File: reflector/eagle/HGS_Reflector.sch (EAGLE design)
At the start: 22 parts, among them J1 U.FL, U1 TQP3M9037, U2 TQP3M903X, U3 LP2985XX-N

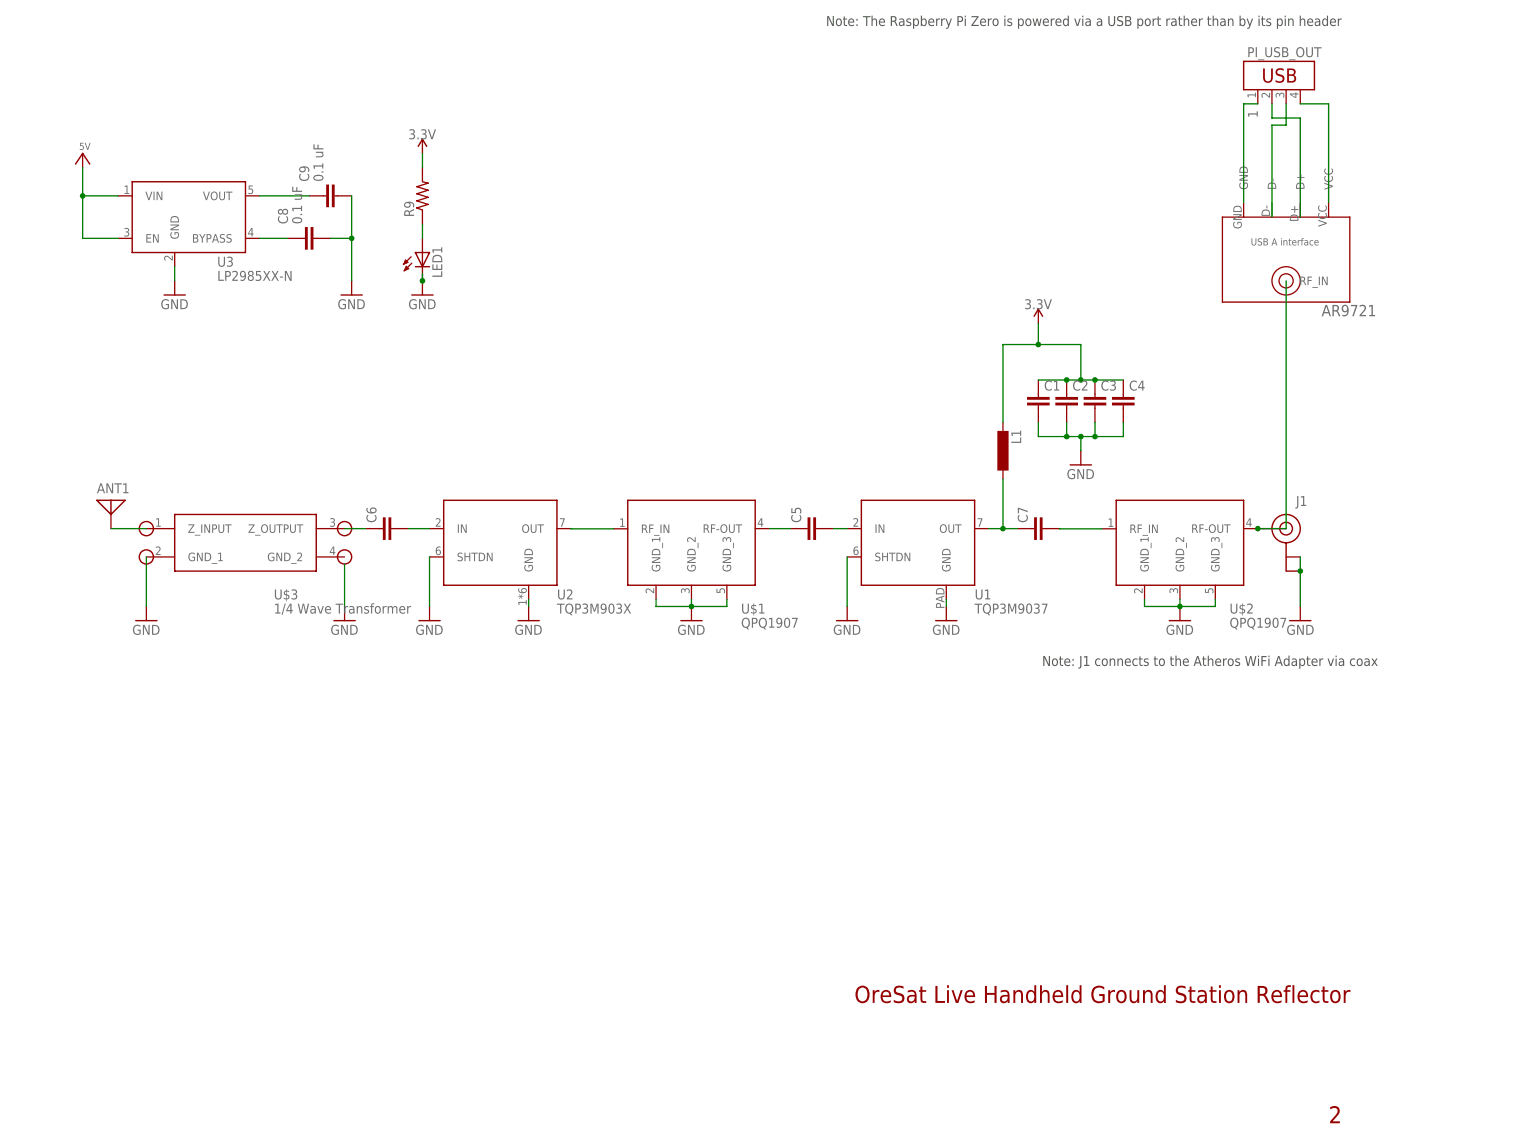
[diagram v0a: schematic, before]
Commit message: Schematic, board and BOM updates
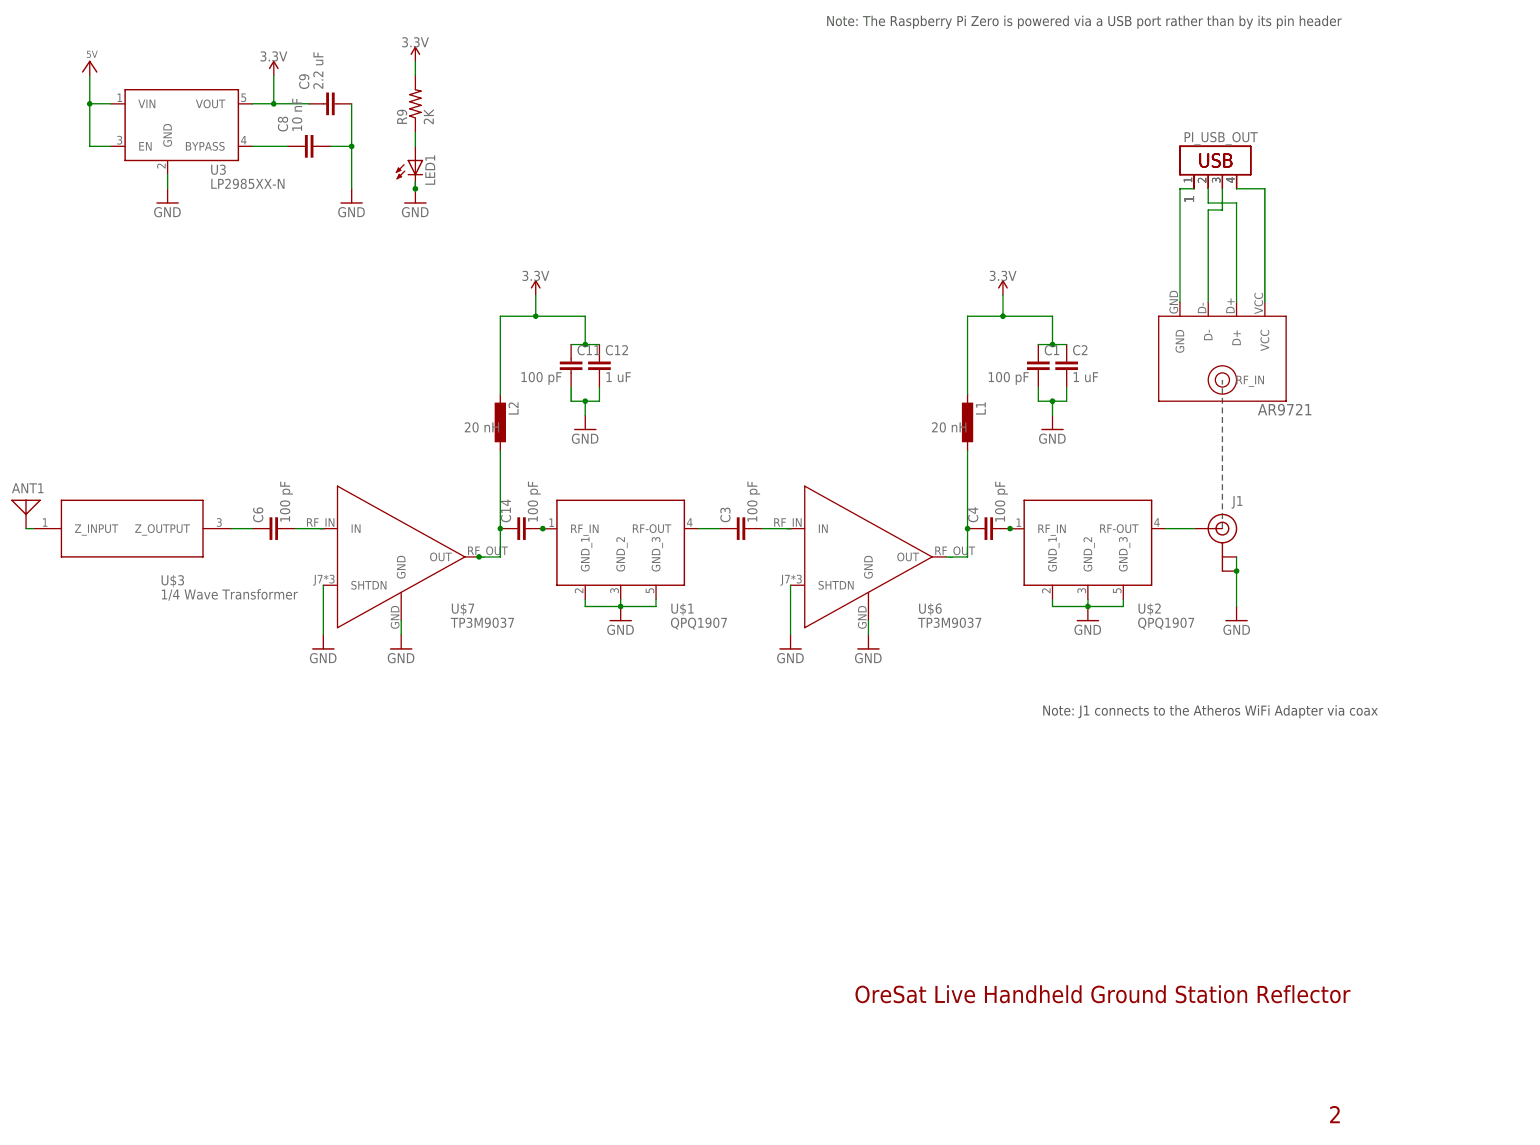
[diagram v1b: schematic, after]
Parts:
- removed C5, C7: (no value), oresat-rcl:C-EU0402-C-NOSILK
- removed U1: TQP3M9037, U-Qorvo-TQP3M9037-LNA:TQP3M9037
- removed U2: TQP3M903X, U-Qorvo-TQP3M903x-LNA:TQP3M903X
- added C11: 100 pF, oresat-rcl:C-EU0603-C-NOSILK
- added C12: 1 uF, oresat-rcl:C-EU0603-C-NOSILK
- added C14: 100 pF, oresat-rcl:C-EU0402-C-NOSILK
- added L2: (no value), rcl:L-EUL3216C
- added PI_USB_OUT1: (no value), con-amp:USB-787616
- added U$6, U$7: LNA-TP3M9037, HGS_Data_Parts:LNA-TP3M9037
- C1, C6: value (none) -> 100 pF
- C2: value (none) -> 1 uF
- C3, C4: value (none) -> 100 pF; device oresat-rcl:C-EU0603-C-NOSILK -> oresat-rcl:C-EU0402-C-NOSILK
- C8: value 0.1 uF -> 10 nF
- C9: value 0.1 uF -> 2.2 uF
- L1: SPICEPREFIX (none) -> 20 nH
- R9: value (none) -> 2K
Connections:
- removed net N$13: C9.1, U3.VOUT
- removed net N$14: PI_USB_OUT.3, U$4.D-
- removed net N$15: PI_USB_OUT.4
- removed net N$7: C5.1, U$1.RF-OUT
- new net N$16: C14.1, L2.1, U$7.OUT
- new net N$18: PI_USB_OUT.2, PI_USB_OUT1.2, U$4.D+
- new net N$19: PI_USB_OUT.3, PI_USB_OUT1.3, U$4.D-
- new net VCC: PI_USB_OUT.4, PI_USB_OUT1.4, U$4.VCC
- net 1: now also PI_USB_OUT1.1, U$4.GND
- net 3.3V: now also C11.1, C12.1, C9.1, L2.2, U3.VOUT; no longer C3.1, C4.1
- net GND: now also C11.2, C12.2, U$6.GND, U$6.SHTDN, U$7.GND, U$7.SHTDN; no longer C3.2, C4.2, U$3.GND_1, U1.GND, U1.SHTDN, U2.GND, U2.SHTDN
- net N$11: now also U$7.IN; no longer U2.IN
- net N$2: now also C4.1, L1.1, U$6.OUT; no longer J1.SIGNAL, U$2.RF-OUT, U$4.RF_IN
- net N$3: now also C4.2; no longer C7.2, U$2.RF_IN
- net N$4: now also C3.1, U$1.RF-OUT; no longer C5.2, U1.IN
- net N$5: now also J1.SIGNAL, U$2.RF-OUT; no longer C7.1, L1.1, U1.OUT
- net N$6: now also C14.2; no longer PI_USB_OUT.2, U$4.D+
- net N$8: now also C3.2, U$6.IN; no longer U$1.RF_IN, U2.OUT
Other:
- moved on the sheet: ANT1, C1, C2, C3, C4, C6, C8, C9, J1, L1, LED1, PI_USB_OUT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
